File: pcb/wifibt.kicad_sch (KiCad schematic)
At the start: 12 parts, among them U901 RTL8723BS, X901 32.768kHz

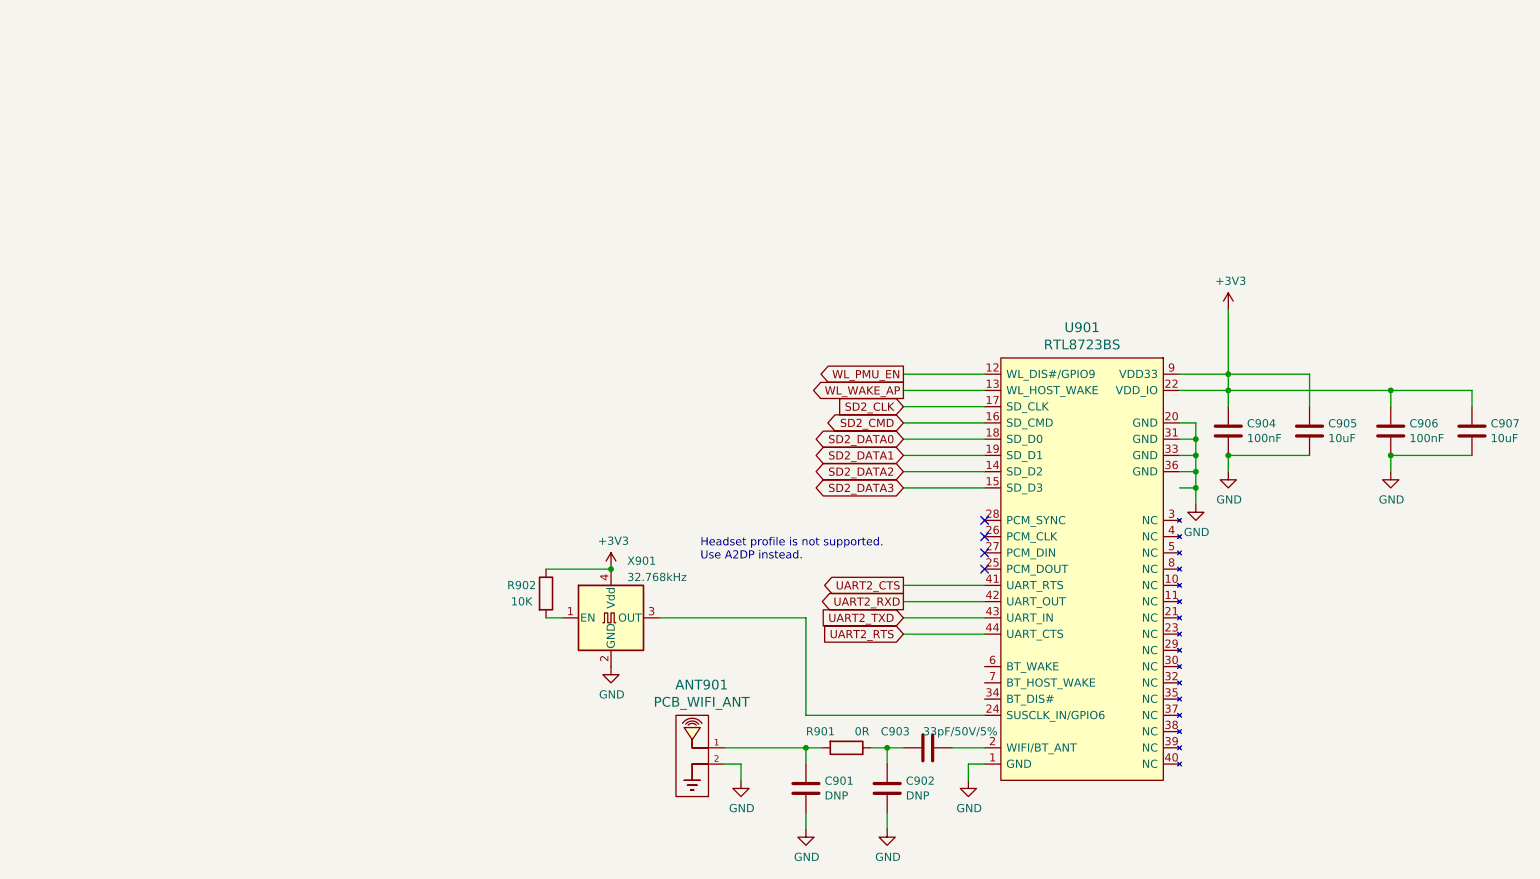
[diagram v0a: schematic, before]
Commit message: pcb: getting ready for r0.2 production
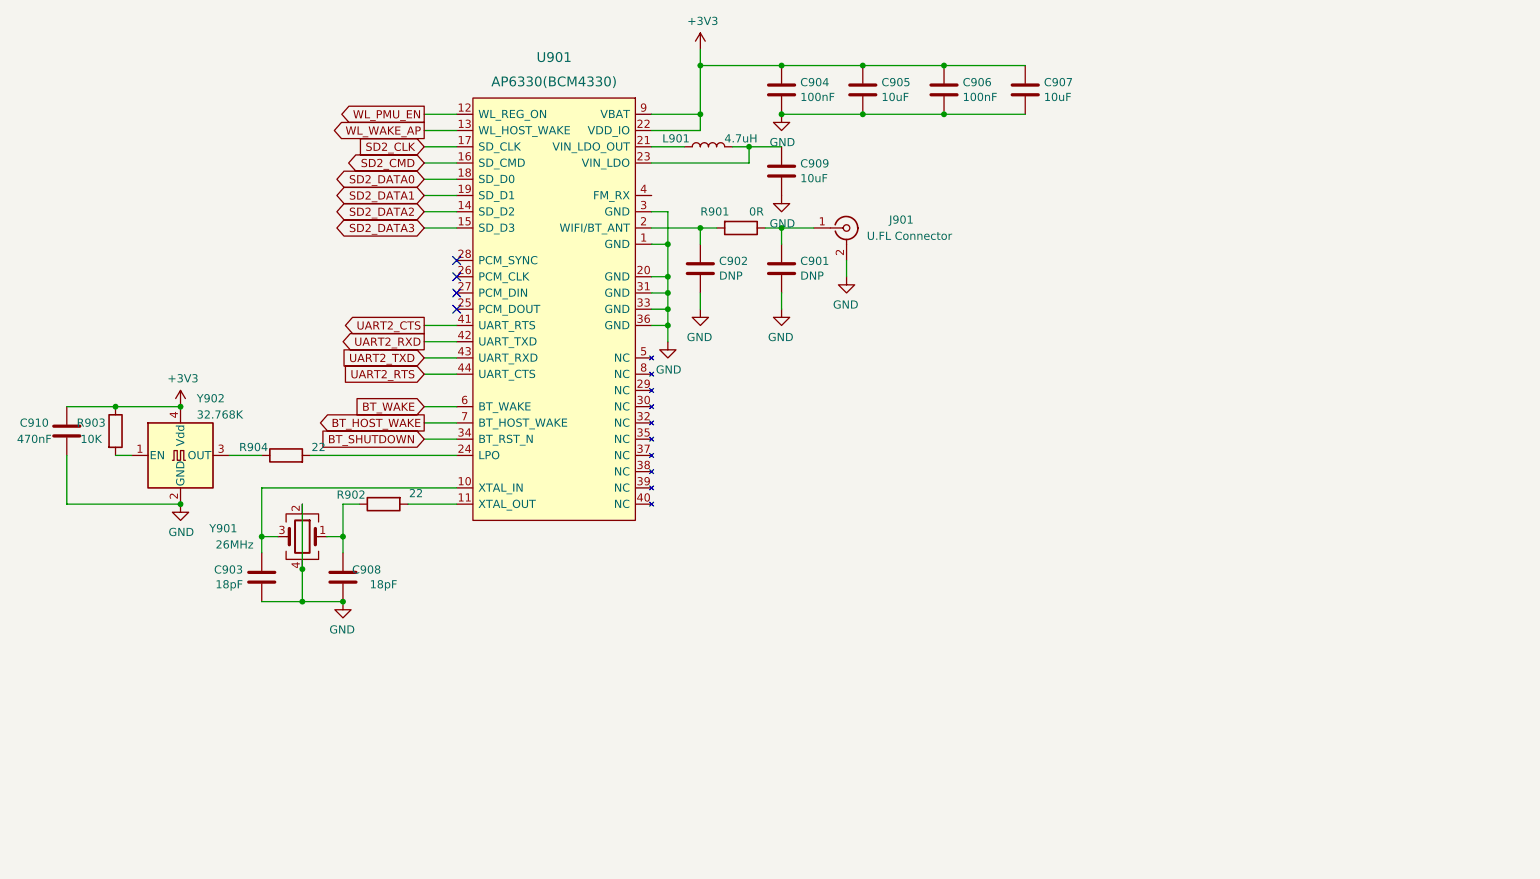
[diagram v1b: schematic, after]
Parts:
- removed ANT901: PCB_WIFI_ANT, footprints:bt_antenna_1ant_2gnd, symbol symbols:WIFI_ANT_ESP8266
- removed U901: RTL8723BS, footprints:RL-SM02BD(RTL8723BS), symbol symbols:RTL8723BS
- removed X901: 32.768kHz, Oscillator:Oscillator_SMD_Abracon_ASE-4Pin_3.2x2.5mm, symbol Oscillator:ASE-xxxMHz
- added C908: 18pF, Capacitor_SMD:C_0402_1005Metric, symbol Device:C
- added C909: 10uF, Capacitor_SMD:C_0603_1608Metric, symbol Device:C
- added C910: 470nF, Capacitor_SMD:C_0402_1005Metric, symbol Device:C
- added J901: U.FL Connector, Connector_Coaxial:U.FL_Molex_MCRF_73412-0110_Vertical, symbol Connector:Conn_Coaxial
- added L901: 4.7uH, footprints:L_1212, symbol Device:L
- added R903: 10K, Capacitor_SMD:C_0402_1005Metric, symbol Device:R
- added R904: 22, Capacitor_SMD:C_0402_1005Metric, symbol Device:R
- added U901: AP6330(BCM4330), footprints:RL-SM02BD(RTL8723BS), symbol symbols:AP6330(BCM4330)
- added Y901: 26MHz, Oscillator:Oscillator_SMD_Abracon_ASE-4Pin_3.2x2.5mm, symbol Device:Crystal_GND24
- added Y902: 32.768K, Oscillator:Oscillator_SMD_Abracon_ASE-4Pin_3.2x2.5mm, symbol Oscillator:ASE-xxxMHz
- C903: value 33pF/50V/5% -> 18pF
- R902: value 10K -> 22
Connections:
- net +3V3: now also C910.2, R903.1, U901.22 (VDD_IO), U901.9 (VBAT), Y902.4 (Vdd); no longer R902.1
- net GND: now also C903.2, C908.2, C909.2, C910.1, J901.2 (Ext), U901.1 (GND), U901.20 (GND), U901.3 (GND), U901.31 (GND), U901.33 (GND), U901.36 (GND), Y901.2, Y901.4, Y902.2 (GND)
- net SD2_CLK: now also U901.17 (SD_CLK)
- net SD2_CMD: now also U901.16 (SD_CMD)
- net SD2_DATA0: now also U901.18 (SD_D0)
- net SD2_DATA1: now also U901.19 (SD_D1)
- net SD2_DATA2: now also U901.14 (SD_D2)
- net SD2_DATA3: now also U901.15 (SD_D3)
- net UART2_CTS: now also U901.41 (UART_RTS)
- net UART2_RTS: now also U901.44 (UART_CTS)
- net UART2_RXD: now also U901.42 (UART_TXD)
- net UART2_TXD: now also U901.43 (UART_RXD)
- net WL_PMU_EN: now also U901.12 (WL_REG_ON)
- net WL_WAKE_AP: now also U901.13 (WL_HOST_WAKE)
- net at C901.2: now also R901.1, J901.1 (In); no longer R901.2
- net at R902.2: now also U901.11 (XTAL_OUT)
- net at C903.1: now also U901.10 (XTAL_IN), Y901.3
- new net: C902.2, R901.2, U901.2 (WIFI/BT_ANT)
- new net: R903.2, Y902.1 (EN)
- new net: R904.1, Y902.3 (OUT)
- new net: C908.1, R902.1, Y901.1
- new net: C909.1, L901.2, U901.23 (VIN_LDO)
- new net: R904.2, U901.24 (LPO)
- new net: L901.1, U901.21 (VIN_LDO_OUT)
- new net BT_HOST_WAKE: U901.7 (BT_HOST_WAKE)
- new net BT_SHUTDOWN: U901.34 (BT_RST_N)
- new net BT_WAKE: U901.6 (BT_WAKE)
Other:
- note removed: "Headset profile is not supported. Use A2DP instead."
- moved on the sheet: C901, C902, C904, C905, C906, C907, R901
